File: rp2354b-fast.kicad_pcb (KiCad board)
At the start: 4 copper layers, 70 x 70 mm, 95 parts, among them J1 USB_C_Receptacle_USB2.0_16P, J2 TC2030-Tag, J3 Batt-Con, J4 MSD-10-C, J5 STPR_OUT, J6 Conn_01x03_Socket, J7 Conn_01x06, J9 Conn_02x06_Odd_Even, SW1 BOOT, SW2 RUN, U1 RP2354B, U11 SX1262, U2 TPS63061, U3 USBLC6-2P6, U4 BMP581, U5 TLV75801PDRV, U6 TLV75533PDRV, U7 DRV8461SPWP, U8 ISM6HG256X, U9 MMC5983MA, Y1 12MHz

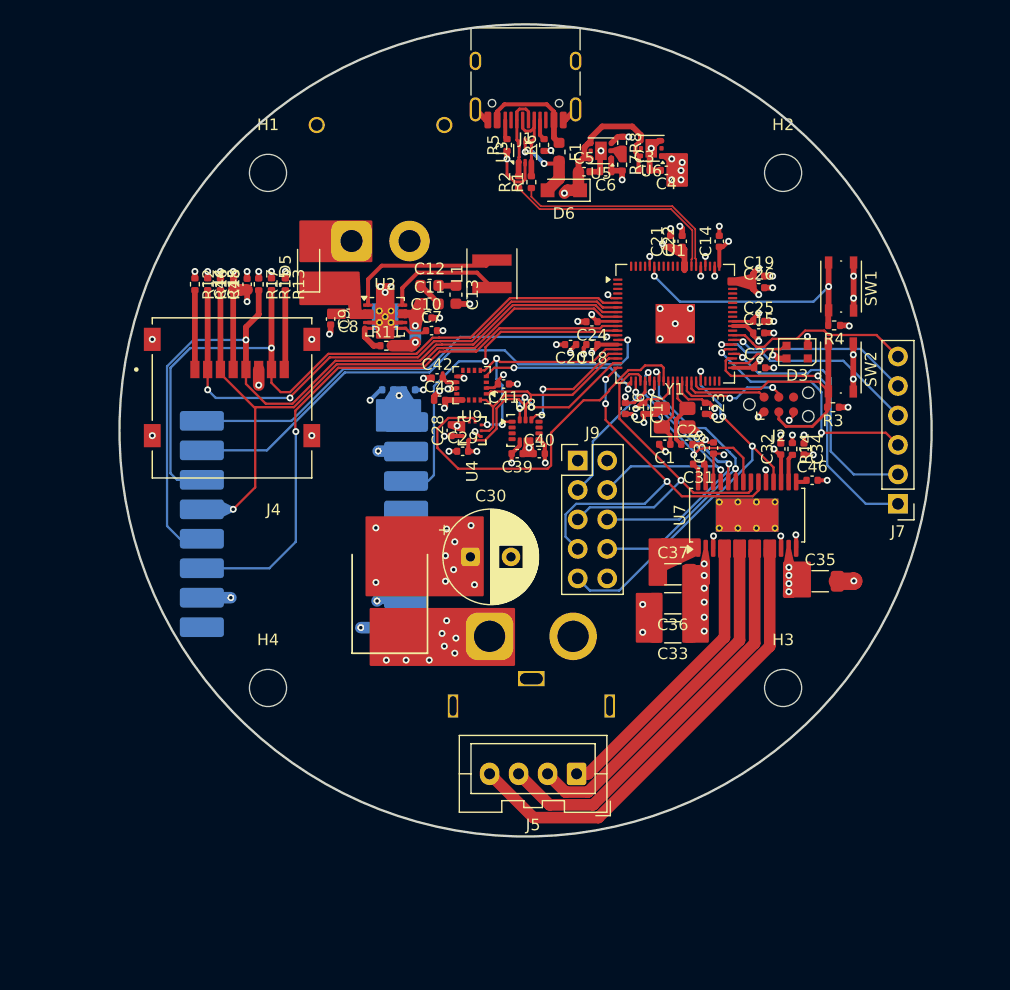
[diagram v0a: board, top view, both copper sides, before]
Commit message: autoroute lol
prob have to move stuff if i wanted to actually do this
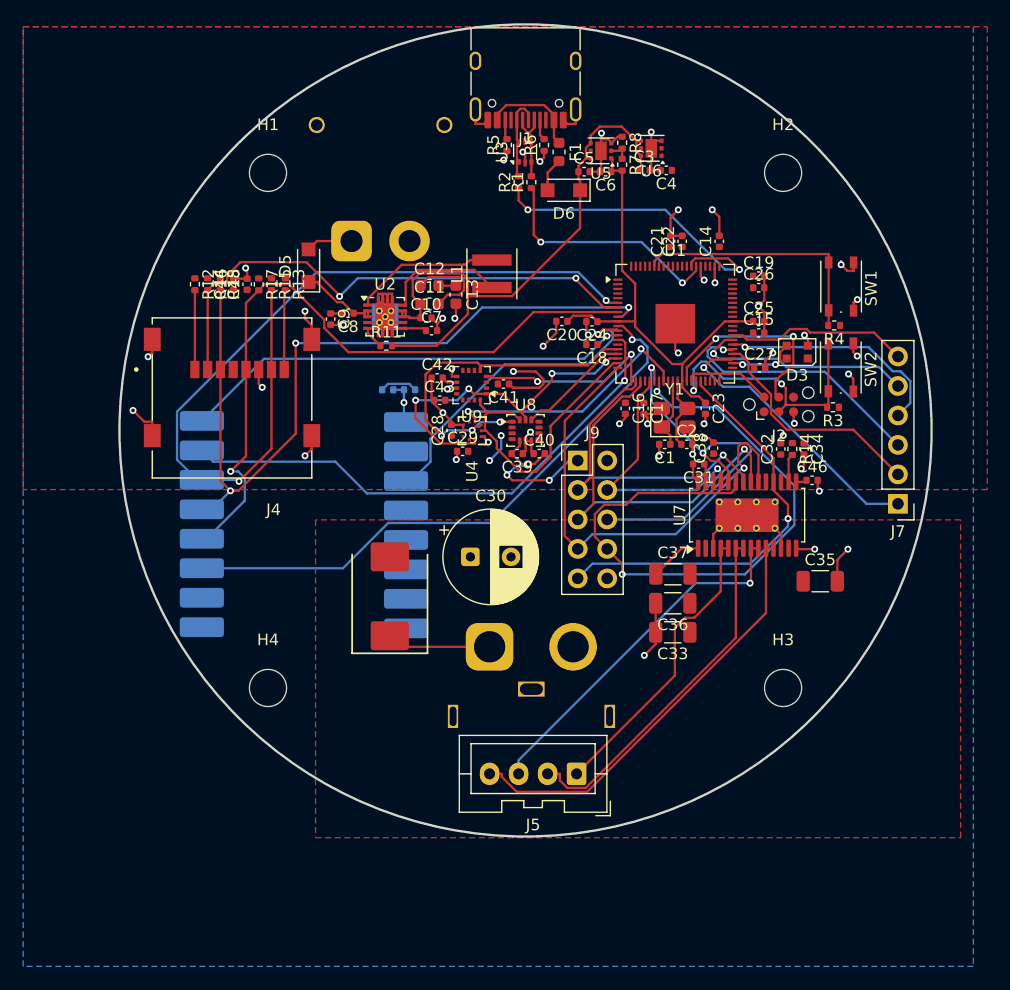
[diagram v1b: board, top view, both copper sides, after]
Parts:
- moved C20 2.14 mm to (140.6, 107.6)
- moved J6 0.90 mm to (134.4, 135.7)
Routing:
- net GND: track 77.6 -> 130.3 mm, vias 73 -> 48
- net +3V3: track 65.1 -> 20.6 mm, vias 40 -> 6
- net /STPER_STEP: track 28.0 -> 55.9 mm
- net +DVDD: track 54.3 -> 39.9 mm, vias 5 -> 0
- net V_OUT: track 38.7 -> 51.0 mm, vias 3 -> 0
- net /GPIO28_CSN_BMP: track 32.4 -> 22.1 mm, vias 0 -> 2
- net /GPIO16_SPI0_RX: track 21.5 -> 31.5 mm
- net /GPIO10_SPI1_SCK: track 70.0 -> 60.5 mm
- net /STPER_DIR: track 24.9 -> 34.1 mm
- net Net-(J6-Pin_1): track 0.00 -> 8.99 mm, vias 8 -> 0
- net /GPIO11_SPI1_TX: track 58.7 -> 67.6 mm, vias 1 -> 3
- net /GPIO08_SPI1_RX: track 63.1 -> 72.0 mm, vias 1 -> 2
- net /USB_DP: track 19.6 -> 27.6 mm, vias 0 -> 2
- net Net-(J2-SWCLK): track 9.94 -> 17.5 mm
- net Net-(D5-K): track 0.00 -> 7.30 mm
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- added copper zone on F.Cu, net +16V8
- added copper zone on F.Cu, net +3V3
- added copper zone on B.Cu, net GND
- removed copper zone on In2.Cu, net +16V8
- removed copper zone on In2.Cu, net +3V3
- removed copper zone on In1.Cu, net GND
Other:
- copper layers 4 -> 2

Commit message: Revert "autoroute lol"
This reverts commit 13dc7621d4bb3c53ef667583583493ebc15fa3aa.
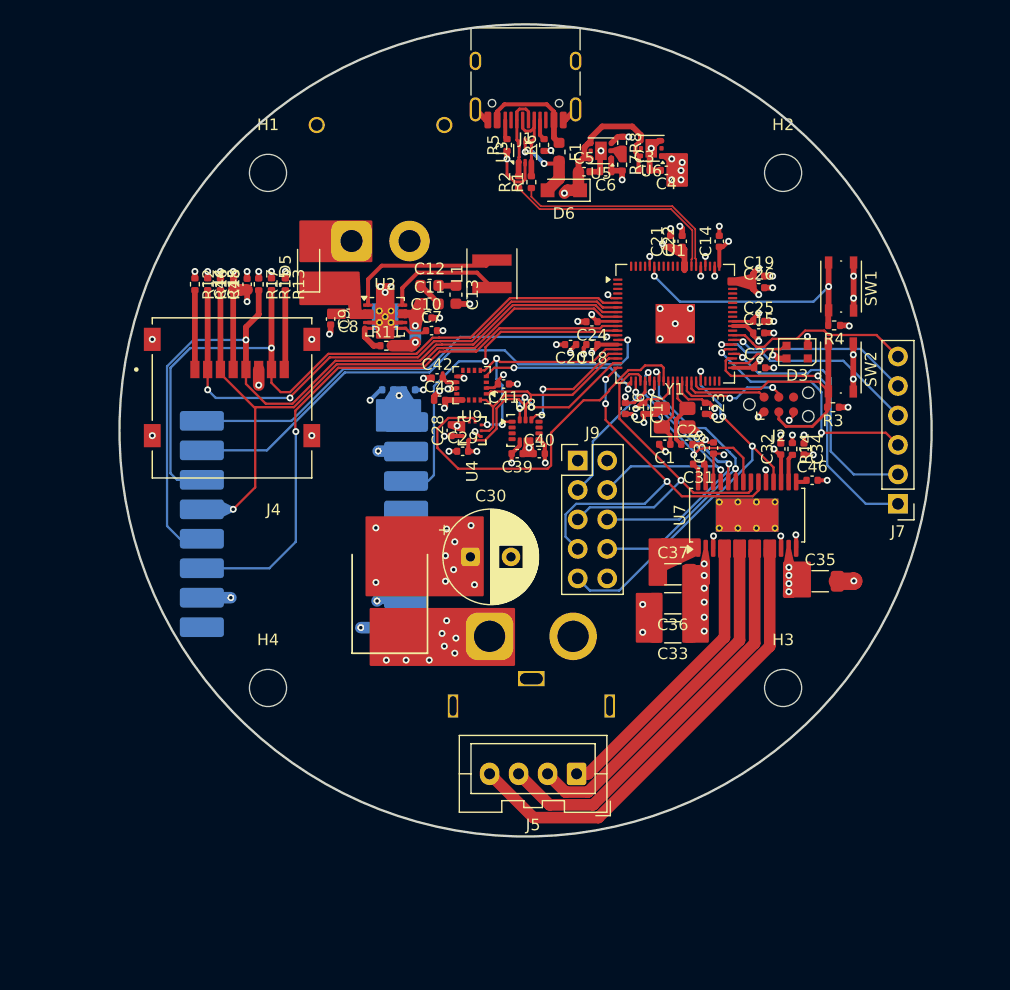
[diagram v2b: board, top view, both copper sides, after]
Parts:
- moved C20 2.14 mm to (141.4, 109.6)
- moved J6 0.90 mm to (134.4, 134.8)
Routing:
- net GND: track 130.3 -> 77.6 mm, vias 48 -> 73
- net +3V3: track 20.6 -> 65.1 mm, vias 6 -> 40
- net /STPER_STEP: track 55.9 -> 28.0 mm
- net +DVDD: track 39.9 -> 54.3 mm, vias 0 -> 5
- net V_OUT: track 51.0 -> 38.7 mm, vias 0 -> 3
- net /GPIO28_CSN_BMP: track 22.1 -> 32.4 mm, vias 2 -> 0
- net /GPIO16_SPI0_RX: track 31.5 -> 21.5 mm
- net /GPIO10_SPI1_SCK: track 60.5 -> 70.0 mm
- net /STPER_DIR: track 34.1 -> 24.9 mm
- net Net-(J6-Pin_1): track 8.99 -> 0.00 mm, vias 0 -> 8
- net /GPIO11_SPI1_TX: track 67.6 -> 58.7 mm, vias 3 -> 1
- net /GPIO08_SPI1_RX: track 72.0 -> 63.1 mm, vias 2 -> 1
- net /USB_DP: track 27.6 -> 19.6 mm, vias 2 -> 0
- net Net-(J2-SWCLK): track 17.5 -> 9.94 mm
- net Net-(D5-K): track 7.30 -> 0.00 mm
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- added copper zone on In2.Cu, net +16V8
- added copper zone on In2.Cu, net +3V3
- added copper zone on In1.Cu, net GND
- removed copper zone on F.Cu, net +16V8
- removed copper zone on F.Cu, net +3V3
- removed copper zone on B.Cu, net GND
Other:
- copper layers 2 -> 4
